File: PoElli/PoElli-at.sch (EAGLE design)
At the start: 85 parts, among them J1 DF12-60DP, T1 POE-ISOLATION, U3 NCP1117, X1 RJ45MOLEX

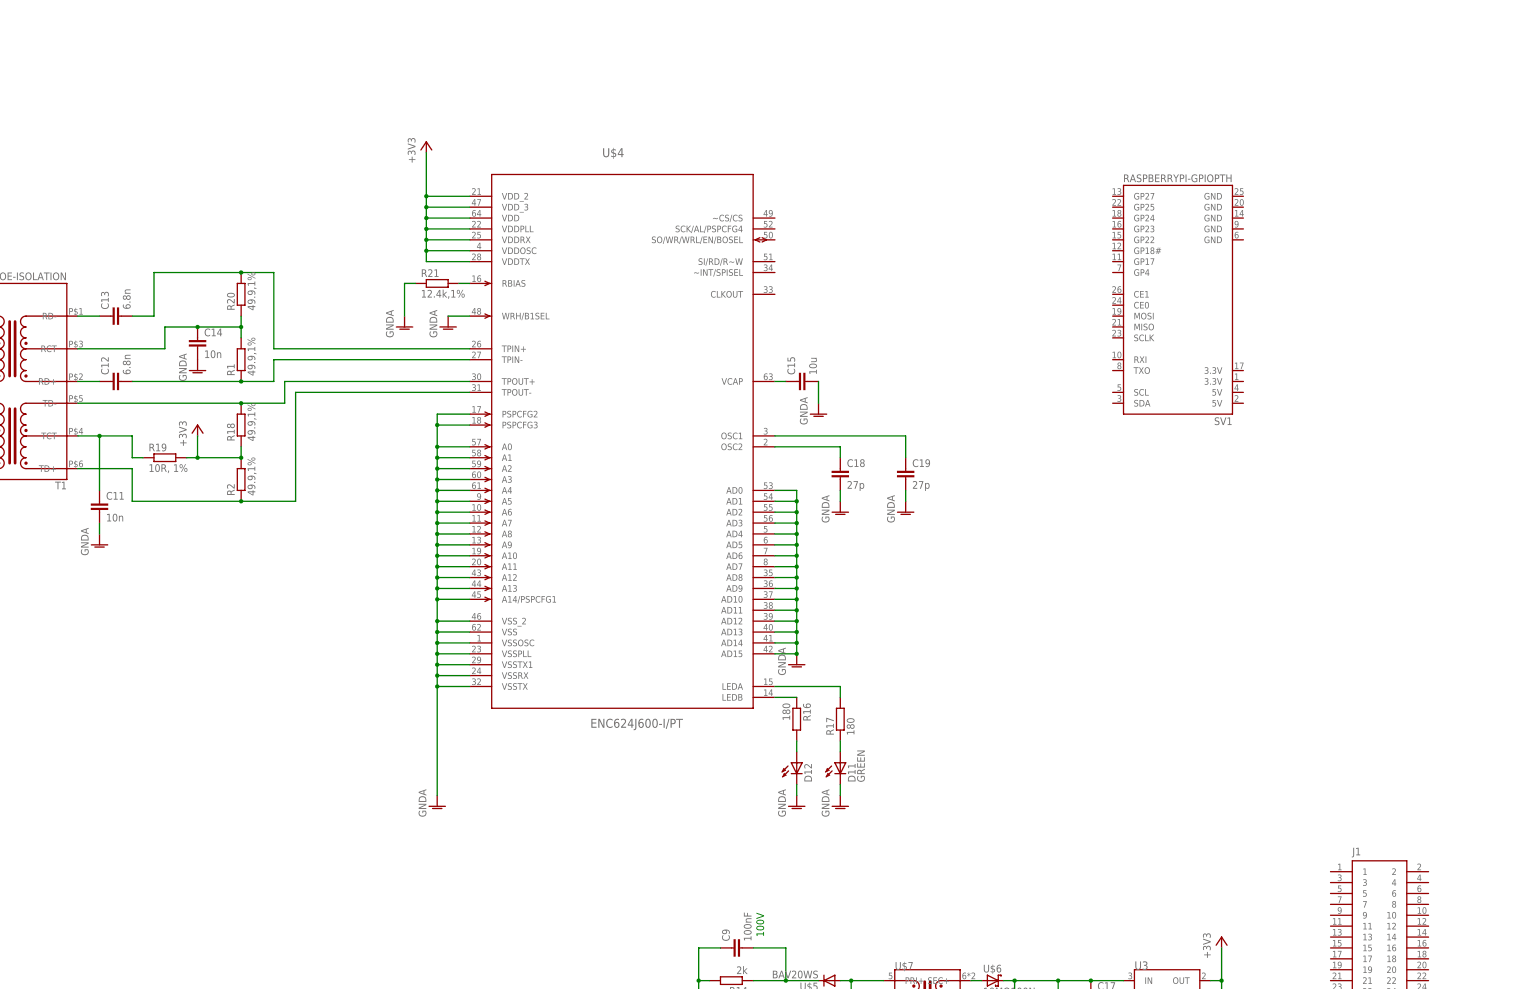
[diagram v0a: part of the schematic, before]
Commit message: Add mux
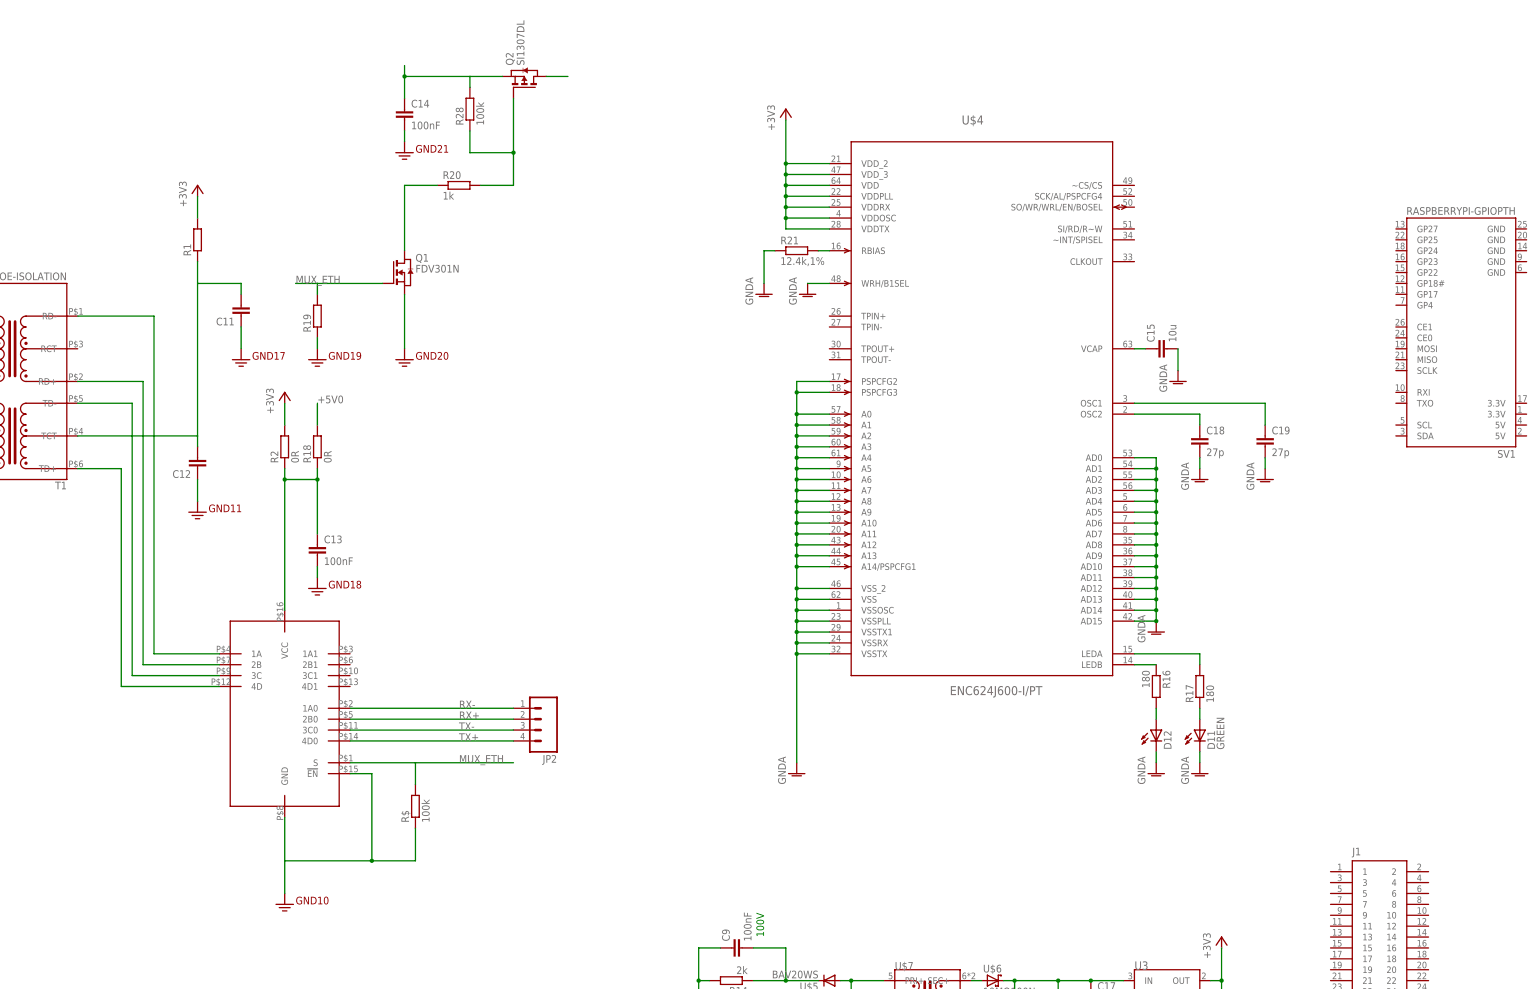
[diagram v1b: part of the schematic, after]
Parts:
- added JP2: (no value), SparkFun-Connectors:M04LOCK
- added Q1: FDV301N, ELL-i-DIscreteSemi:FDV301N
- added Q2: SI1307DL, ELL-i-DIscreteSemi:SI1307DL
- added R$, R28: 100k, ELL-i-Passives:R0805
- added U1: FST3257, ELL-i-DigitalIC:FST3257
- C11: value 10n -> (none); device ELL-i-Passives:C0603 -> ELL-i-Passives:C0805
- C12: value 6.8n -> (none); device ELL-i-Passives:C0603 -> ELL-i-Passives:C0805
- C13: value 6.8n -> 100nF; device ELL-i-Passives:C0603 -> ELL-i-Passives:C0805
- C14: value 10n -> 100nF; device ELL-i-Passives:C0603 -> ELL-i-Passives:C0805
- R1: value 49.9,1% -> (none); device ELL-i-Passives:R0603 -> ELL-i-Passives:R0805
- R18, R2: value 49.9,1% -> 0R; device ELL-i-Passives:R0603 -> ELL-i-Passives:R0805
- R19: value 10R, 1% -> (none); device ELL-i-Passives:R0603 -> ELL-i-Passives:R0805
- R20: value 49.9,1% -> 1k; device ELL-i-Passives:R0603 -> ELL-i-Passives:R0805
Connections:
- removed net +3V3: C16.+, R18.1, R19.2, R2.2, U$4.VDD, U$4.VDDOSC, U$4.VDDPLL, U$4.VDDRX, U$4.VDDTX, U$4.VDD_2, U$4.VDD_3, U3.OUT, U3.TAB
- new net +5V0: C16.+, R1.2, R18.2, R2.2, U$4.VDD, U$4.VDDOSC, U$4.VDDPLL, U$4.VDDRX, U$4.VDDTX, U$4.VDD_2, U$4.VDD_3, U3.OUT, U3.TAB
- new net 3.3V: C11.1, C12.1, C14.2, Q1.S, R19.1
- new net MUX_ETH: Q1.G, R$.2, R19.2, U1.S
- new net N$56: Q1.D, R20.1
- new net N$57: Q2.G, R20.2, R28.1
- new net N$58: C14.1, Q2.S, R28.2
- new net N$60: Q2.D
- new net RX+: JP2.2, U1.2B0
- new net RX-: JP2.1, U1.1A0
- new net TX+: JP2.4, U1.4D0
- new net TX-: JP2.3, U1.3C0
- net GNDA: no longer C11.2, C14.2
- net N$11: now also T1.TD+, U1.4D; no longer C14.1, R1.2, R20.1, T1.RCT
- net N$12: now also T1.TD-, U1.3C; no longer C13.1, T1.RD-
- net N$13: now also T1.RD+, U1.2B; no longer R18.2, T1.TD-, U$4.TPOUT+
- net N$14: now also T1.RD-, U1.1A; no longer R2.1, T1.TD+, U$4.TPOUT-
- net N$39: now also R$.1, U1.!EN, U1.GND; no longer C12.1, T1.RD+
- net N$40: now also C11.2, T1.TCT; no longer U$4.TPIN-
- net N$43: now also C13.1, R18.1, R2.1, U1.VCC; no longer C11.1, R19.1, T1.TCT
- net N$44: no longer R20.2, U$4.TPIN+
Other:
- moved on the sheet: C11, C12, C13, C14, C15, C18, C19, D11, D12, R1, R16, R17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
